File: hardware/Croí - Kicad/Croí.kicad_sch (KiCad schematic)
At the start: 5 parts, among them J1 2060-1452/998-404, J2 ESQ-110-X-X-D, U1 NUP2105LT1G, U2 STM32F411CEUx

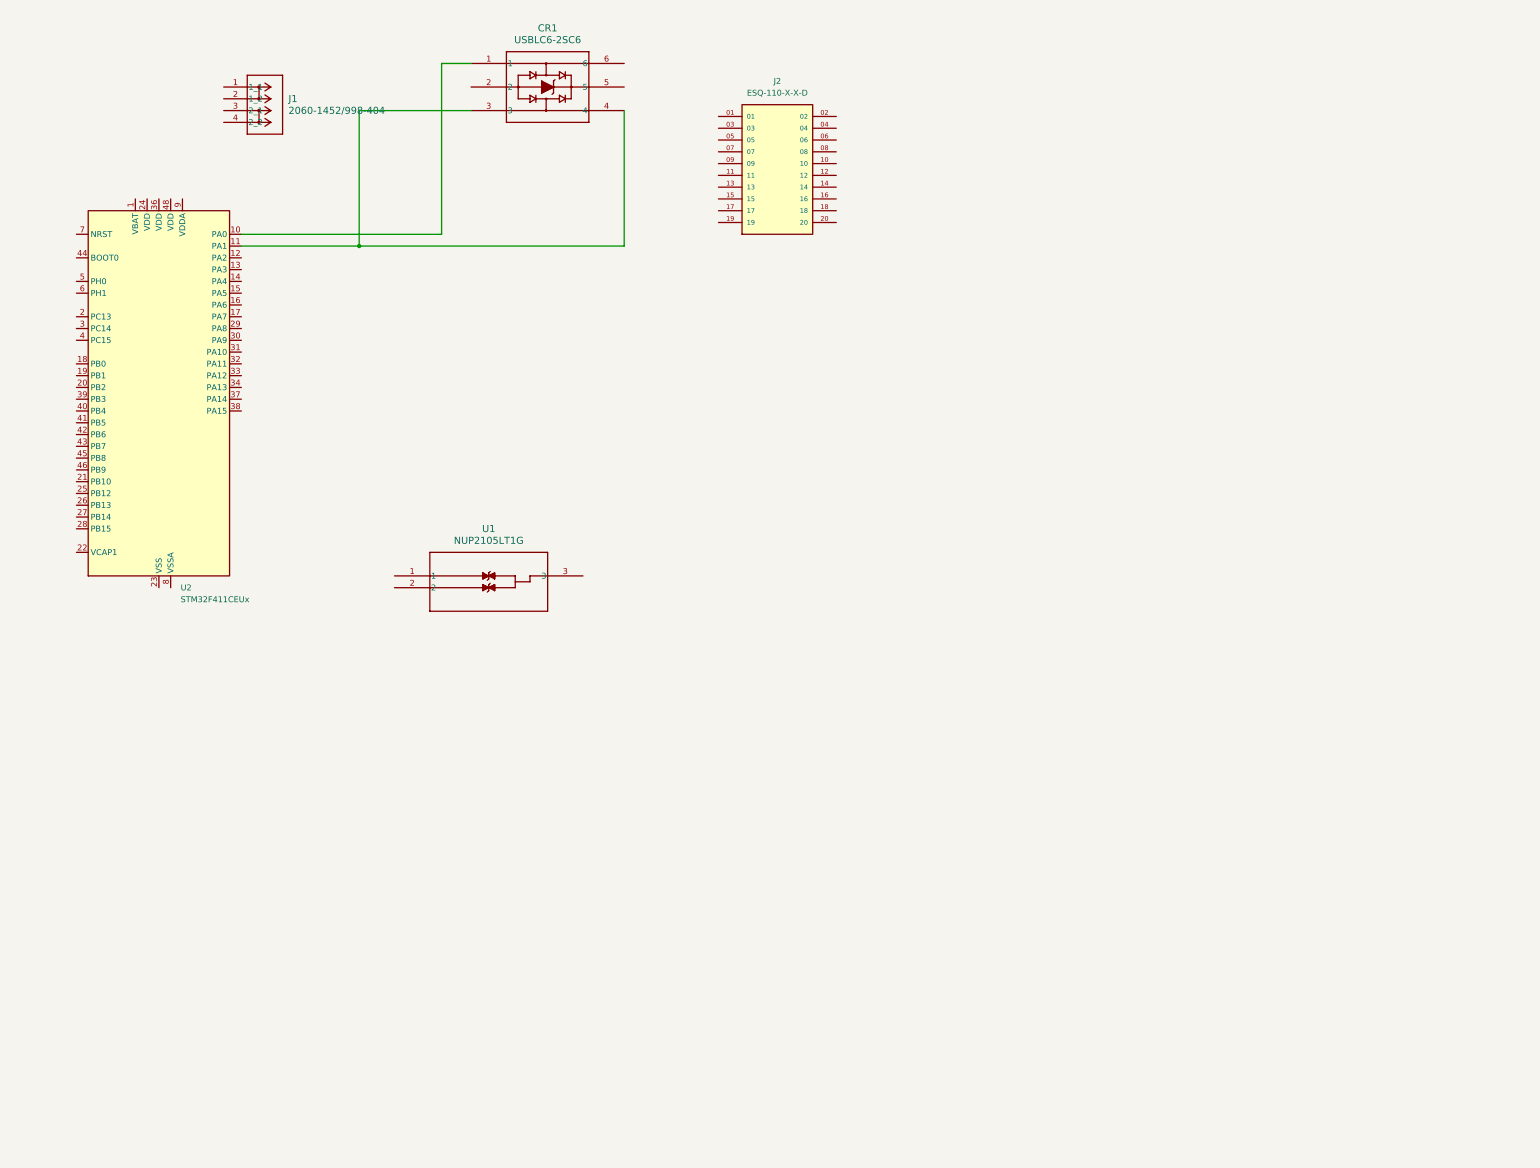
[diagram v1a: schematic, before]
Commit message: did basically all of it
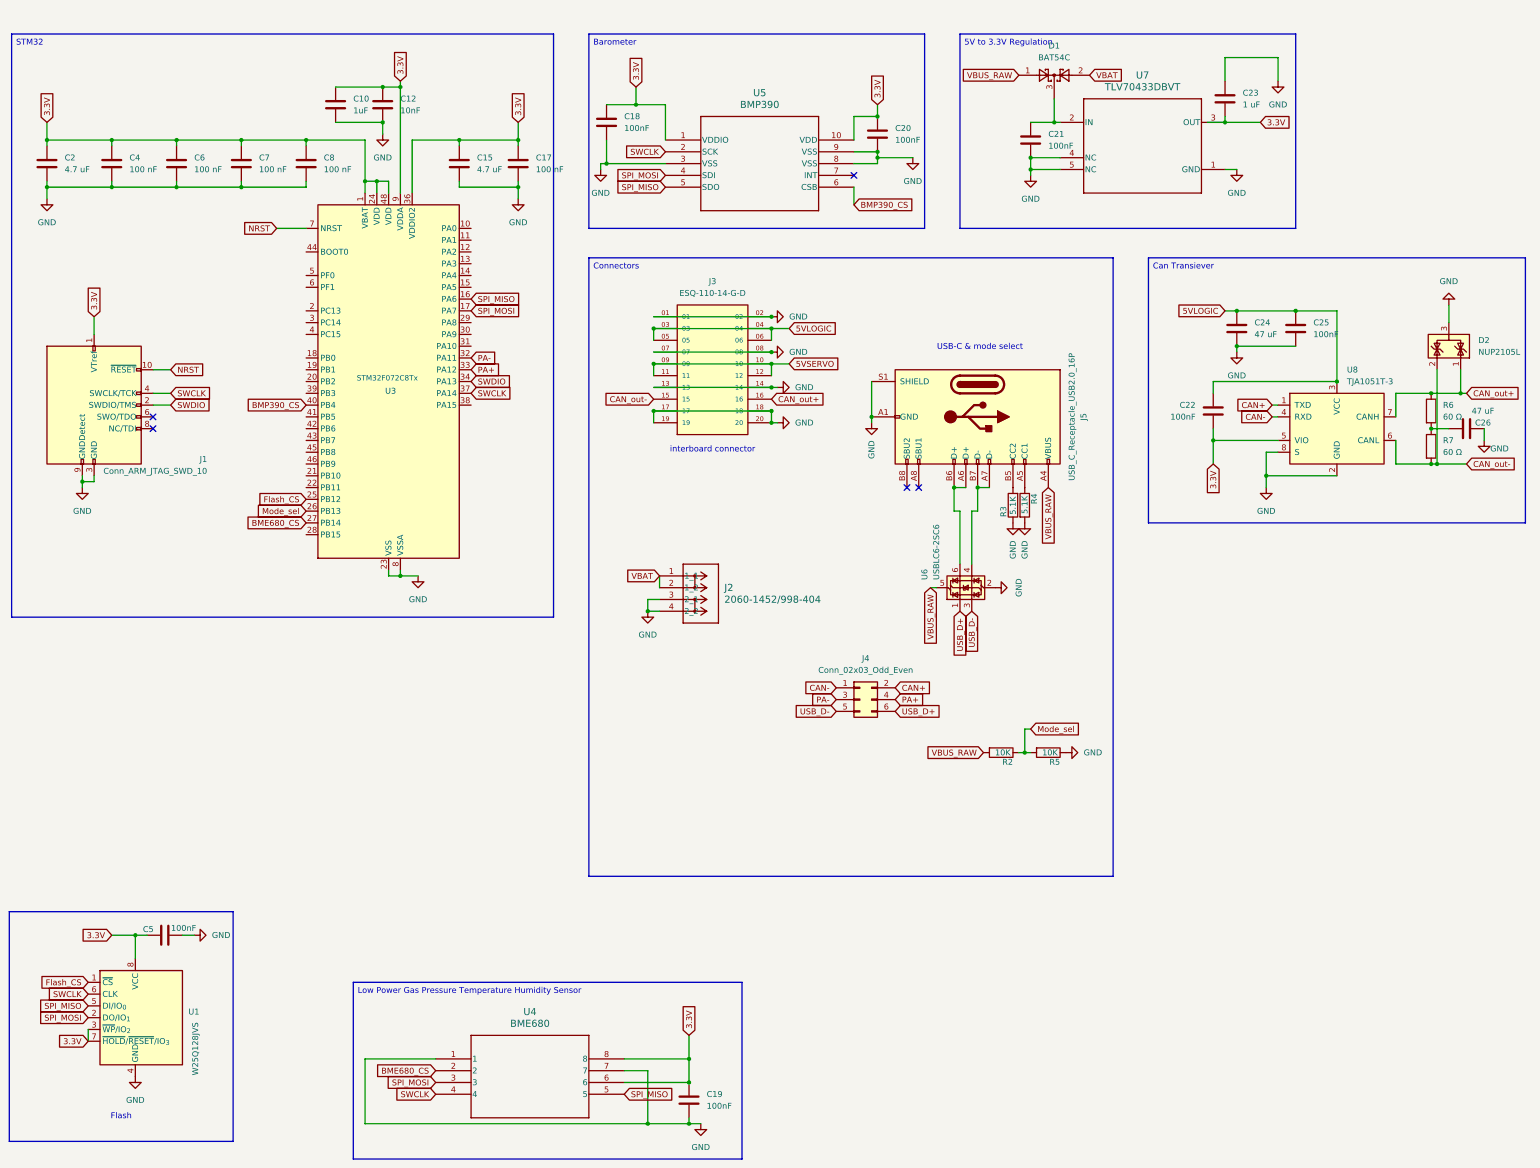
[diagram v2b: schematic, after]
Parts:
- removed CR1: USBLC6-2SC6, SOT23-6L_STM, symbol usb:USBLC6-2SC6
- removed J2: ESQ-110-X-X-D, SAMTEC_ESQ-110-14-G-D, symbol ESQ:ESQ-110-X-X-D
- removed U1: NUP2105LT1G, SOT-23_3L_ONS, symbol 1:NUP2105LT1G
- removed U2: STM32F411CEUx, Package_DFN_QFN:QFN-48-1EP_7x7mm_P0.5mm_EP5.6x5.6mm, symbol MCU_ST_STM32F4:STM32F411CEUx
- added C10: 1uF, Capacitor_SMD:C_0402_1005Metric, symbol Device:C
- added C12: 10nF, Capacitor_SMD:C_0402_1005Metric, symbol Device:C
- added C15, C2: 4.7 uF, Capacitor_SMD:C_0402_1005Metric, symbol Device:C
- added C17, C4, C6, C7, C8: 100 nF, Capacitor_SMD:C_0402_1005Metric, symbol Device:C
- added C18, C19, C20, C21, C22, C25, C5: 100nF, Capacitor_SMD:C_0402_1005Metric, symbol Device:C
- added C23: 1 uF, Capacitor_SMD:C_0402_1005Metric, symbol Device:C
- added C24, C26: 47 uF, Capacitor_SMD:C_0402_1005Metric, symbol Device:C
- added D1: BAT54C, Package_TO_SOT_SMD:SOT-23, symbol Diode:BAT54C
- added D2: NUP2105L, Package_TO_SOT_SMD:SOT-23, symbol Power_Protection:NUP2105L
- added J1: Conn_ARM_JTAG_SWD_10, symbol Connector:Conn_ARM_JTAG_SWD_10
- added J3: ESQ-110-14-G-D, Connector_PinHeader_2.54mm:PinHeader_2x10_P2.54mm_Vertical, symbol ESQ-110-X-X-D:ESQ-110-X-X-D
- added J4: Conn_02x03_Odd_Even, Connector_PinHeader_1.00mm:PinHeader_2x03_P1.00mm_Vertical, symbol Connector_Generic:Conn_02x03_Odd_Even
- added J5: USB_C_Receptacle_USB2.0_16P, Connector_USB:USB_C_Receptacle_G-Switch_GT-USB-7010ASV, symbol Connector:USB_C_Receptacle_USB2.0_16P
- added R2, R5: 10K, Resistor_SMD:R_0402_1005Metric, symbol Device:R
- added R3, R4: 5.1K, Resistor_SMD:R_0402_1005Metric, symbol Device:R
- added R6, R7: 60 Ω, Resistor_SMD:R_0402_1005Metric, symbol Device:R
- added U1: W25Q128JVS, Package_SO:SOIC-8_5.3x5.3mm_P1.27mm, symbol Memory_Flash:W25Q128JVS
- added U3: STM32F072C8Tx, Package_QFP:LQFP-48_7x7mm_P0.5mm, symbol MCU_ST_STM32F0:STM32F072C8Tx
- added U4: BME680, footprints:LGA8_BME680_BOS, symbol BME680:BME680
- added U5: BMP390, footprints:10LGA_2X2X0p75_BOS, symbol BMP390:BMP390
- added U6: USBLC6-2SC6, Package_TO_SOT_SMD:SOT-23-6, symbol Power_Protection:USBLC6-2SC6
- added U7: TLV70433DBVT, TLV70433DBVT:DBV0005A_N, symbol TLV70433DBVT:TLV70433DBVT
- added U8: TJA1051T-3, Package_SO:SOIC-8_3.9x4.9mm_P1.27mm, symbol Interface_CAN_LIN:TJA1051T-3
- J2: renamed from J1; footprint WAG -> footprints:WAG
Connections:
- net VBAT: now reaches J2.1 (1_1)
- net VBAT: now also J2.2 (1_2), D1.2
- net GND: now reaches J2.3 (2_1)
- net GND: now also J2.4 (2_2), C10.2, C12.2, C15.2, C17.2, C18.2, C19.2, C2.2, C20.2, C21.2, C23.1, C24.2, C25.2, C26.2, C4.2, C5.2, C6.2, C7.2, C8.2, D2.3 (A), J1.3 (GND), J1.5 (GND), J1.9 (GNDDetect), J3.01, J3.02, J3.07, J3.08, J3.13, J3.14, J3.17, J3.18, J3.19, J3.20, J5.A1 (GND), J5.A12 (GND), J5.B1 (GND), J5.B12 (GND), J5.S1 (SHIELD), R3.1, R4.2, R5.1, U1.4 (GND), U3.23 (VSS), U3.35 (VSS), U3.47 (VSS), U3.8 (VSSA), U4.1, U4.7, U5.3 (VSS), U5.8 (VSS), U5.9 (VSS), U6.2 (GND), U7.1 (GND), U7.4 (NC), U7.5 (NC), U8.2 (GND), U8.8 (S)
- new net: C21.1, D1.3, U7.2 (IN)
- new net: J5.A7 (D-), J5.B7 (D-), U6.4 (I/O2)
- new net: J5.A6 (D+), J5.B6 (D+), U6.6 (I/O1)
- new net: J5.B5 (CC2), R3.2
- new net: C26.1, R6.2, R7.1
- new net: J5.A5 (CC1), R4.1
- new net 3.3V: C10.1, C12.1, C15.1, C17.1, C18.1, C19.1, C2.1, C20.1, C22.1, C23.2, C4.1, C5.1, C6.1, C7.1, C8.1, J1.1 (VTref), U1.3 (~{WP}/IO_{2}), U1.7 (~{HOLD}/~{RESET}/IO_{3}), U1.8 (VCC), U3.1 (VBAT), U3.24 (VDD), U3.36 (VDDIO2), U3.48 (VDD), U3.9 (VDDA), U4.6, U4.8, U5.1 (VDDIO), U5.10 (VDD), U7.3 (OUT), U8.5 (VIO)
- new net 5VLOGIC: C22.2, C24.1, C25.1, J3.03, J3.04, J3.05, J3.06, U8.3 (VCC)
- new net 5VSERVO: J3.09, J3.10, J3.11, J3.12
- new net BME680_CS: U3.27 (PB14), U4.2
- new net BMP390_CS: U3.40 (PB4), U5.6 (CSB)
- new net CAN+: J4.2 (Pin_2), U8.1 (TXD)
- new net CAN-: J4.1 (Pin_1), U8.4 (RXD)
- new net CAN_out+: D2.1 (K), J3.16, R6.1, U8.7 (CANH)
- new net CAN_out-: D2.2 (K), J3.15, R7.2, U8.6 (CANL)
- new net Flash_CS: U1.1 (~{CS}), U3.25 (PB12)
- new net Mode_sel: R2.1, R5.2, U3.26 (PB13)
- new net NRST: J1.10 (~{RESET}), U3.7 (NRST)
- new net PA+: J4.4 (Pin_4), U3.33 (PA12)
- new net PA-: J4.3 (Pin_3), U3.32 (PA11)
- new net SPI_MISO: U1.5 (DI/IO_{0}), U3.16 (PA6), U4.5, U5.5 (SDO)
- new net SPI_MOSI: U1.2 (DO/IO_{1}), U3.17 (PA7), U4.3, U5.4 (SDI)
- new net SWCLK: J1.4 (SWCLK/TCK), U1.6 (CLK), U3.37 (PA14), U4.4, U5.2 (SCK)
- new net SWDIO: J1.2 (SWDIO/TMS), U3.34 (PA13)
- new net USB_D+: J4.6 (Pin_6), U6.1 (I/O1)
- new net USB_D-: J4.5 (Pin_5), U6.3 (I/O2)
- new net VBUS_RAW: D1.1, J5.A4 (VBUS), J5.A9 (VBUS), J5.B4 (VBUS), J5.B9 (VBUS), R2.2, U6.5 (VBUS)
- no-connect marks 0 -> 5
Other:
- note added: "Flash"
- note added: "USB-C & mode select"
- note added: "interboard connector"
- moved on the sheet: J2
